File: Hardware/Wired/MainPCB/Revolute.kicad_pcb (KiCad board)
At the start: 4 copper layers, 16.8 x 10.7 mm, 32 parts, among them J1 USB_A, U1 nRF52840_aQFN73, U3 AP2112K-3.3, U4 debug_ports, X1 32MHZ, X2 32.768 kHz

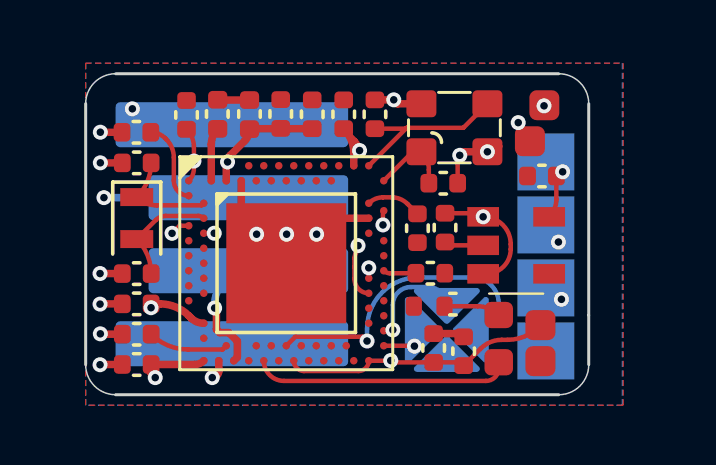
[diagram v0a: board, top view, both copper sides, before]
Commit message: current version
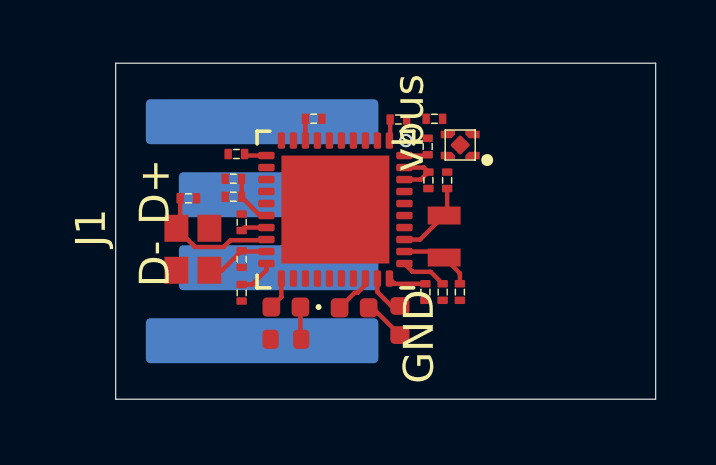
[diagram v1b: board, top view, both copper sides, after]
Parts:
- removed ? (x4): , 
- removed C14: 1uF, Capacitor_SMD:C_0402_1005Metric
- removed C18: 12pF, Capacitor_SMD:C_0402_1005Metric
- removed C20, C21: 4.7uF, Capacitor_SMD:C_0402_1005Metric
- removed L3: 15nH, Inductor_SMD:L_0402_1005Metric
- removed U3: AP2112K-3.3, Package_TO_SOT_SMD:SOT-23-5
- removed U4: debug_ports, Library:Debug pin cluster
- added C3: 12pF, Library:Capacitor-0201, F.Cu at (178.1, 85.9)
- added C4: 100nF, Library:Capacitor-0201, F.Cu at (177.9, 89.6)
- added L1: 10uH, Inductor_SMD:L_0402_1005Metric, F.Cu at (176.5, 90.6)
- added U2: MIC5504, Library:TDFN-4, F.Cu at (178.5, 84.7)
- C1: value 12pF -> 4.7uF; footprint Capacitor_SMD:C_0402_1005Metric -> Library:Capacitor-0201
- C10, C13, C2: footprint Capacitor_SMD:C_0402_1005Metric -> Library:Capacitor-0201
- C11: value 100pF -> 100nF; footprint Capacitor_SMD:C_0402_1005Metric -> Library:Capacitor-0201
- C12: value 100nF -> 820pF; footprint Capacitor_SMD:C_0402_1005Metric -> Library:Capacitor-0201
- C15, C16: value 1uF -> 12pF; footprint Capacitor_SMD:C_0402_1005Metric -> Library:Capacitor-0201
- C17: value 12pF -> 100pF; footprint Capacitor_SMD:C_0402_1005Metric -> Library:Capacitor-0201
- C5, C7: value 100nF -> 4.7uF; footprint Capacitor_SMD:C_0402_1005Metric -> Library:Capacitor-0201
- C6: value 4.7uF -> 1uF; footprint Capacitor_SMD:C_0402_1005Metric -> Library:Capacitor-0201
- C8: value 100nF -> 1uF; footprint Capacitor_SMD:C_0402_1005Metric -> Library:Capacitor-0201
- C9: value 820pF -> 1uF; footprint Capacitor_SMD:C_0402_1005Metric -> Library:Capacitor-0201
- D1: footprint Library:LED_0603_1608Metric-nosilk -> LED_SMD:LED_0402_1005Metric
- L2: value 10uH -> 15nH
- U1: value nRF52840_aQFN73 -> nrf52833_qfn40; footprint Library:AQFN-73-1EP_7x7mm_P0.5mm_NRF52840-custom -> Library:QFN-40-1EP_5x5mm_P0.4mm_EP3.6x3.6mm
- X1: value 32MHZ -> 32.768 kHz; footprint Library:crystal 32mhz -> Library:Crystal_SMD_2012-2Pin_2.0x1.2mm
- X2: value 32.768 kHz -> 32MHZ; footprint Crystal:Crystal_SMD_2012-2Pin_2.0x1.2mm -> Library:Crystal_SMD_2016-4Pin_2.0x1.6mm
- moved C16 11.8 mm to (169.4, 86.5)
- moved J1 11.2 mm to (175.8, 87.6)
- moved C6 10.6 mm to (177.4, 85.9), turned to -90 degrees
- moved C5 9.72 mm to (177.4, 84.8), turned to 90 degrees
- moved C7 8.02 mm to (176.4, 83.9), turned to 180 degrees
- moved L2 7.89 mm to (175.0, 90.2), turned to 0 degrees
- moved C8 7.64 mm to (177.6, 83.9), turned to 0 degrees
- moved C9 7.28 mm to (170.9, 85.9)
- moved D1 7.17 mm to (172.7, 90.1), turned to 180 degrees
- moved C2 6.57 mm to (178.5, 89.6)
- moved C11 6.24 mm to (171.2, 89.7), turned to -90 degrees
- moved C15 5.37 mm to (171.2, 88.5)
- moved R1 4.90 mm to (172.7, 91.2)
- moved C1 4.82 mm to (173.6, 83.9)
- moved C17 4.02 mm to (171.2, 87.3), turned to -90 degrees
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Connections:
- C1 pad 2: Net-(U1-XC1) -> VDD_nRF
- C11 pad 1: GND -> VDD_nRF
- C11 pad 2: Net-(U1-DEC3) -> GND
- C12 pad 1: VDD_nRF -> GND
- C12 pad 2: GND -> Net-(U1-DEC5)
- C13 pad 1: VBUS -> VDD_nRF
- C15 pad 1: Net-(U1-DEC4) -> GND
- C15 pad 2: GND -> Net-(U1-XC2)
- C16 pad 1: VDD_nRF -> GND
- C16 pad 2: GND -> Net-(U1-XC1)
- C17 pad 1: Net-(U1-XL1/P0.00) -> GND
- C17 pad 2: GND -> Net-(U1-DEC3)
- C2 pad 1: GND -> Net-(U1-P0.00/XL1)
- C2 pad 2: Net-(U1-XC2) -> GND
- C5 pad 1: Net-(U1-DEC1) -> VBUS
- C6 pad 1: GND -> VDD_nRF
- C6 pad 2: VDD_nRF -> GND
- C7 pad 2: VDD_nRF -> Net-(U1-DECUSB)
- C8 pad 1: GND -> VBUS
- C8 pad 2: VDD_nRF -> GND
- C9 pad 1: GND -> Net-(U1-DEC4)
- C9 pad 2: Net-(U1-DEC5) -> GND
- J1 pad 2: Net-(J1-D-) -> D-
- J1 pad 3: Net-(J1-D+) -> D+
- L2 pad 1: Net-(L2-Pad1) -> Net-(U1-DEC4)
- L2 pad 2: Net-(U1-DCC) -> Net-(L1-Pad1)
- X1 pad 1: Net-(U1-XC1) -> Net-(U1-P0.00/XL1)
- X1 pad 2: GND -> Net-(U1-P0.01/XL2)
- X2 pad 1: Net-(U1-XL1/P0.00) -> Net-(U1-XC1)
- X2 pad 2: Net-(U1-XL2/P0.01) -> GND
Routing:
- net VBUS: track 30.0 -> 0.79 mm, vias 3 -> 0
- net GND: track 17.6 -> 0.00 mm, vias 12 -> 1
- net P0.26: track 14.3 -> 0.00 mm, vias 2 -> 0
- net Net-(J1-D-): track 12.8 -> 0.00 mm, vias 2 -> 0
- net P0.27: track 12.7 -> 0.00 mm, vias 2 -> 0
- net VDD_nRF: track 17.1 -> 5.01 mm, vias 5 -> 0
- net P1.05: track 10.9 -> 0.00 mm, vias 2 -> 0
- net Net-(U1-P0.18/~{RESET}): track 10.4 -> 0.00 mm, vias 1 -> 0
- net P1.07: track 10.2 -> 0.00 mm, vias 2 -> 0
- net BLUE_LED: track 8.61 -> 1.09 mm
- net Net-(U1-DEC4): track 10.4 -> 3.08 mm, vias 2 -> 0
- net Net-(J1-D+): track 4.14 -> 0.00 mm, vias 1 -> 0
- net Net-(U1-XL2/P0.01): track 3.83 -> 0.00 mm
- net Net-(U1-XC2): track 5.88 -> 2.18 mm
- net Net-(U1-XL1/P0.00): track 3.61 -> 0.00 mm
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- removed copper zone on B.Cu, net GND
- removed copper zone on F.Cu, net GND
- removed copper zone on In1.Cu, net GND
- removed copper zone on In2.Cu, net VDD_nRF
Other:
- board size 16.8 x 10.7 mm -> 18 x 11.2 mm
